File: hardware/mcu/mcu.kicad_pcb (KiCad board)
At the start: 2 copper layers, 24.5 x 68.8 mm, 61 parts, among them J1 TYPE-C-31-M-12, J2 Conn_01x11, J3 Conn_01x11, J4 JST-PH Battery, J5 n_log, Q1 MUN5214DW1T1G, Q2 SI2301CDS-T1-GE3, Q3 SI2301CDS-T1-GE3, Q4 SI2301CDS-T1-GE3, SW1 Reset, SW2 REG SELECT, SW3 Boot, U1 ESP32-PICO-D4, U2 CP210x, U3 USBLC6-2SC6, U4 TP4065, U5 ME6210A33P, U6 TPS630x1

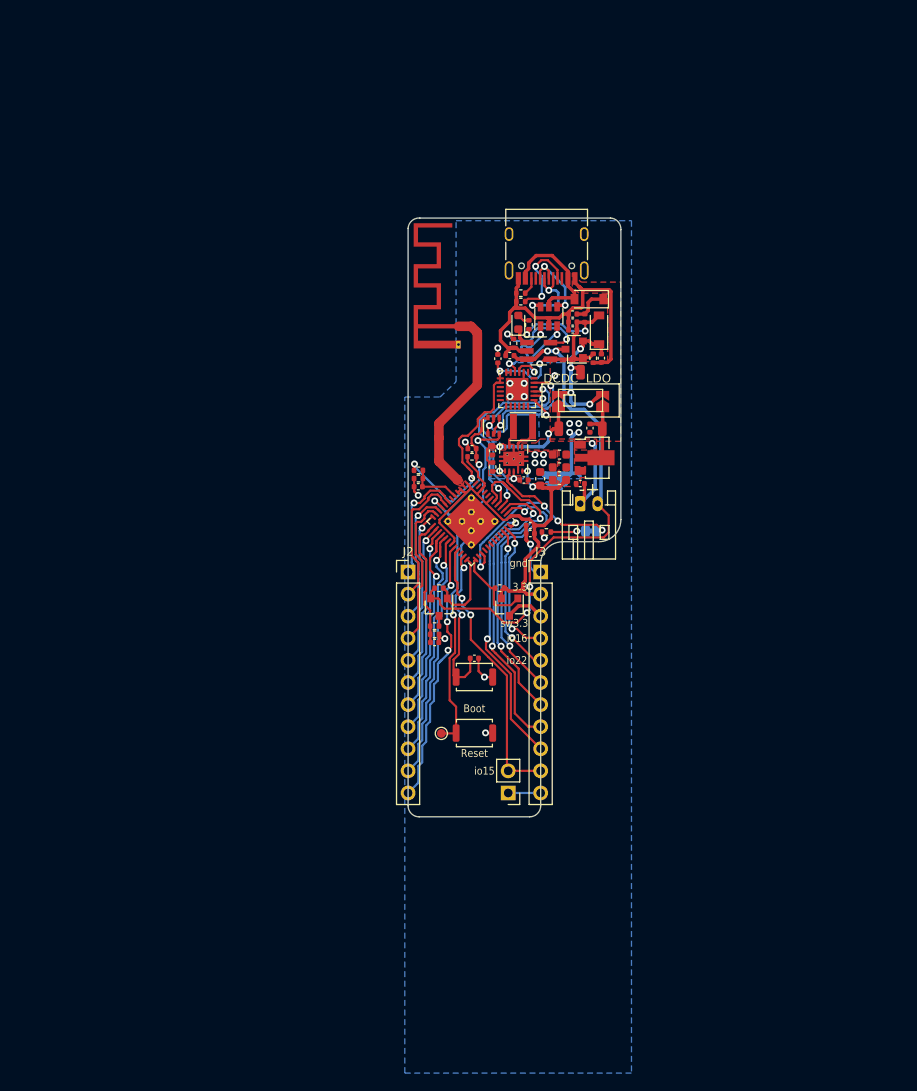
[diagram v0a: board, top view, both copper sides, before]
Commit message: Prototype scale v0.1
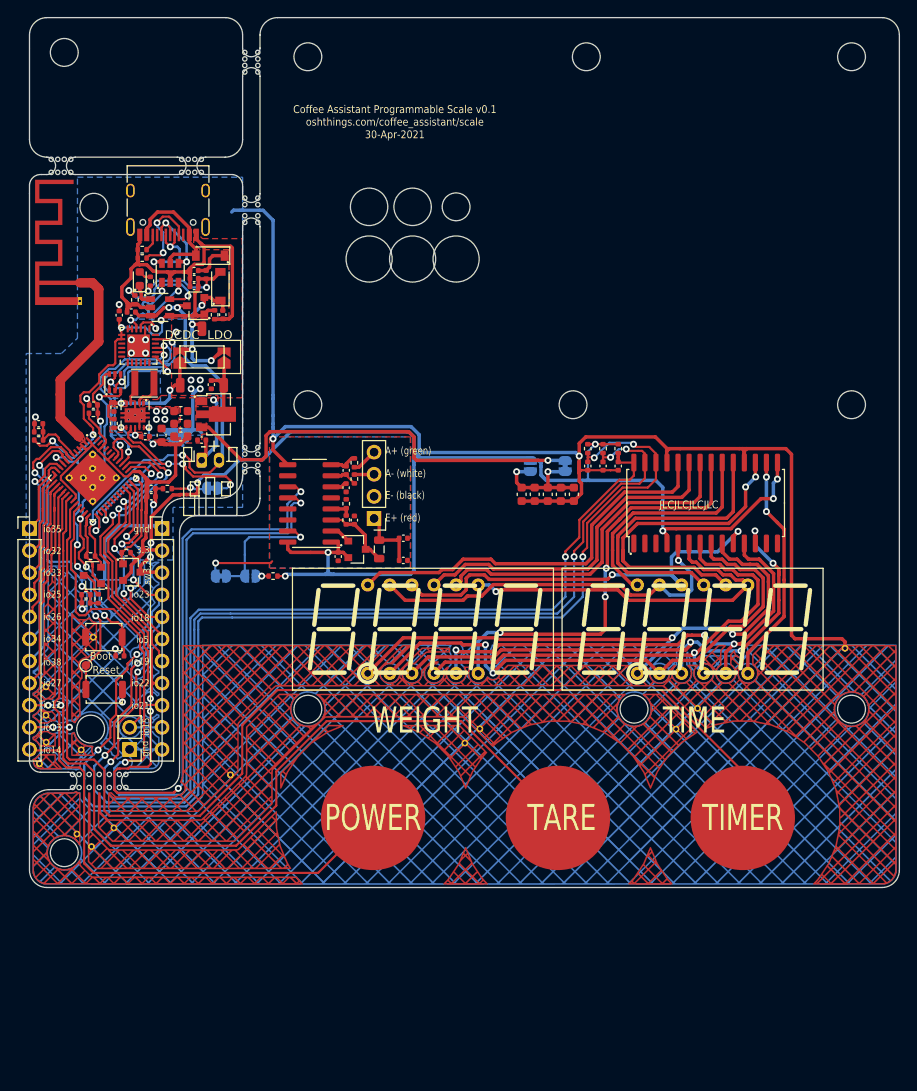
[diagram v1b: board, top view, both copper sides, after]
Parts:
- added C21: 10uF, Capacitor_SMD:C_0402_1005Metric, F.Cu at (93.5, 105.0)
- added C22: 10uF, Capacitor_SMD:C_0402_1005Metric, F.Cu at (95.3, 100.8)
- added C23: 100nF, Capacitor_SMD:C_0402_1005Metric, F.Cu at (94.4, 97.0)
- added C24: 100nF, Capacitor_SMD:C_0402_1005Metric, F.Cu at (94.4, 95.0)
- added C25: 100pF, Capacitor_SMD:C_0402_1005Metric, F.Cu at (122.2, 94.5)
- added C26: 100pF, Capacitor_SMD:C_0402_1005Metric, F.Cu at (123.9, 94.5)
- added C27: 100pF, Capacitor_SMD:C_0402_1005Metric, F.Cu at (125.7, 94.5)
- added C28: 22uF, Capacitor_SMD:C_0603_1608Metric, F.Cu at (119.1, 97.8)
- added C29: 22uF, Capacitor_SMD:C_0603_1608Metric, F.Cu at (114.6, 97.8)
- added C30: 22uF, Capacitor_SMD:C_0603_1608Metric, F.Cu at (117.6, 97.8)
- added C31: 22uF, Capacitor_SMD:C_0603_1608Metric, F.Cu at (120.6, 97.8)
- added C32: 22uF, Capacitor_SMD:C_0603_1608Metric, F.Cu at (116.1, 97.8)
- added C33: 100nF, Capacitor_SMD:C_0402_1005Metric, F.Cu at (101.0, 102.8)
- added C34: 10uF, Capacitor_SMD:C_0402_1005Metric, F.Cu at (101.0, 105.4)
- added CAP1: Power, custom:CapTouch_12mm, F.Cu at (97.5, 135.0)
- added CAP2: Tare, custom:CapTouch_12mm, F.Cu at (118.8, 135.0)
- added CAP3: Timer/Cal, custom:CapTouch_12mm, F.Cu at (140.0, 135.0)
- added CAP_GND_HATCHED_1: Cap sense grid ground, scale:cap_gnd_1_hatched, F.Cu at (65.7, 117.5)
- added CAP_GND_HATCHED_2: Cap sense grid ground, scale:cap_gnd_2_hatched, F.Cu at (108.0, 128.9)
- added CAP_GND_HATCHED_3: Cap sense grid ground, scale:cap_gnd_3_hatched, F.Cu at (62.0, 118.2)
- added CAP_GND_HATCHED_4: Cap sense grid ground, scale:cap_gnd_4_hatched, F.Cu at (108.0, 128.9)
- added J6: Conn_01x04, Connector_PinHeader_2.54mm:PinHeader_1x04_P2.54mm_Vertical, F.Cu at (97.6, 100.6)
- added JP2: extra_caps_nSwitched, Jumper:SolderJumper-2_P1.3mm_Bridged_RoundedPad1.0x1.5mm, B.Cu at (119.6, 94.5)
- added JP3: extra_caps_switched, Jumper:SolderJumper-2_P1.3mm_Open_RoundedPad1.0x1.5mm, B.Cu at (115.6, 94.5)
- added JP4: 80SPS, Jumper:SolderJumper-2_P1.3mm_Open_RoundedPad1.0x1.5mm, B.Cu at (83.4, 107.2)
- added JP5: 10SPS, Jumper:SolderJumper-2_P1.3mm_Bridged_RoundedPad1.0x1.5mm, B.Cu at (80.0, 107.2)
- added L2: 3.3uH, Inductor_SMD:L_0805_2012Metric, F.Cu at (98.2, 104.1)
- added Q5: SS8550, Package_TO_SOT_SMD:SOT-23, F.Cu at (95.7, 104.1)
- added R15: 100, Resistor_SMD:R_0402_1005Metric, F.Cu at (95.3, 96.0)
- added R16: 100, Resistor_SMD:R_0402_1005Metric, F.Cu at (95.3, 94.2)
- added R17: 20k, Resistor_SMD:R_0402_1005Metric, F.Cu at (94.4, 100.7)
- added R18: 8.2k, Resistor_SMD:R_0402_1005Metric, F.Cu at (94.4, 98.9)
- added R19: 10k, Resistor_SMD:R_0402_1005Metric, F.Cu at (122.2, 92.5)
- added R20: 10k, Resistor_SMD:R_0402_1005Metric, F.Cu at (123.9, 92.5)
- added R21: 10k, Resistor_SMD:R_0402_1005Metric, F.Cu at (125.7, 92.5)
- added R22: 10k, Resistor_SMD:R_0402_1005Metric, F.Cu at (86.0, 107.2)
- added REF**: MountingHole_3.2mm_M3_ISO7380_Pad, MountingHole:MountingHole_3.2mm_M3_ISO7380_Pad, F.Cu at (90.0, 122.5)
- added REF**: MountingHole_3.2mm_M3_ISO7380_Pad, MountingHole:MountingHole_3.2mm_M3_ISO7380_Pad, F.Cu at (65.0, 124.8)
- added REF**: MountingHole_3.2mm_M3_ISO7380_Pad, MountingHole:MountingHole_3.2mm_M3_ISO7380_Pad, F.Cu at (62.0, 139.0)
- added REF**: MountingHole_3.2mm_M3_ISO7380_Pad, MountingHole:MountingHole_3.2mm_M3_ISO7380_Pad, F.Cu at (152.5, 47.5)
- added REF**: MountingHole_3.2mm_M3_ISO7380_Pad, MountingHole:MountingHole_3.2mm_M3_ISO7380_Pad, F.Cu at (90.0, 47.5)
- added REF**: MountingHole_3.2mm_M3_ISO7380_Pad, MountingHole:MountingHole_3.2mm_M3_ISO7380_Pad, F.Cu at (65.4, 64.8)
- added REF**: MountingHole_3.2mm_M3_ISO7380_Pad, MountingHole:MountingHole_3.2mm_M3_ISO7380_Pad, F.Cu at (152.5, 122.5)
- added REF**: MountingHole_3.2mm_M3_ISO7380_Pad, MountingHole:MountingHole_3.2mm_M3_ISO7380_Pad, F.Cu at (127.5, 122.5)
- added REF**: MountingHole_3.2mm_M3_ISO7380_Pad, MountingHole:MountingHole_3.2mm_M3_ISO7380_Pad, F.Cu at (152.5, 87.5)
- added REF**: MountingHole_3.2mm_M3_ISO7380_Pad, MountingHole:MountingHole_3.2mm_M3_ISO7380_Pad, F.Cu at (122.0, 47.5)
- added REF**: MountingHole_3.2mm_M3_ISO7380_Pad, MountingHole:MountingHole_3.2mm_M3_ISO7380_Pad, F.Cu at (120.5, 87.5)
- added REF**: load_cell, custom:load_cell, F.Cu at (126.0, 67.5)
- added REF**: MountingHole_3.2mm_M3_ISO7380_Pad, MountingHole:MountingHole_3.2mm_M3_ISO7380_Pad, F.Cu at (62.0, 47.0)
- added REF**: MountingHole_3.2mm_M3_ISO7380_Pad, MountingHole:MountingHole_3.2mm_M3_ISO7380_Pad, F.Cu at (90.0, 87.5)
- added U10: FJ3461AH, custom:FJ3461AH, F.Cu at (134.2, 113.3)
- added U7: HX711, custom:SOP-16_3.9x9.9mm_P1.27mm, F.Cu at (90.2, 98.8)
- added U8: TM1638, Package_SO:SOIC-28W_7.5x17.9mm_P1.27mm, F.Cu at (135.7, 98.8)
- added U9: FJ3461AH, custom:FJ3461AH, F.Cu at (103.2, 113.3)
- added mouse-bite-single: VAL**, custom:mouse-bite-single, F.Cu at (84.2, 66.5)
- added mouse-bite-single: VAL**, custom:mouse-bite-single, F.Cu at (76.2, 60.8)
- added mouse-bite-single: VAL**, custom:mouse-bite-single, F.Cu at (75.5, 60.8)
- added mouse-bite-single: VAL**, custom:mouse-bite-single, F.Cu at (77.0, 59.3)
- added mouse-bite-single: VAL**, custom:mouse-bite-single, F.Cu at (76.2, 59.3)
- added mouse-bite-single: VAL**, custom:mouse-bite-single, F.Cu at (68.3, 130.0)
- added mouse-bite-single: VAL**, custom:mouse-bite-single, F.Cu at (68.3, 131.5)
- added mouse-bite-single: VAL**, custom:mouse-bite-single, F.Cu at (62.8, 59.3)
- added mouse-bite-single: VAL**, custom:mouse-bite-single, F.Cu at (62.8, 60.8)
- added mouse-bite-single: VAL**, custom:mouse-bite-single, F.Cu at (61.2, 59.3)
- added mouse-bite-single: VAL**, custom:mouse-bite-single, F.Cu at (60.5, 59.3)
- added mouse-bite-single: VAL**, custom:mouse-bite-single, F.Cu at (84.2, 65.8)
- added mouse-bite-single: VAL**, custom:mouse-bite-single, F.Cu at (62.0, 60.8)
- added mouse-bite-single: VAL**, custom:mouse-bite-single, F.Cu at (61.2, 60.8)
- added mouse-bite-single: VAL**, custom:mouse-bite-single, F.Cu at (60.5, 60.8)
- added mouse-bite-single: VAL**, custom:mouse-bite-single, F.Cu at (62.0, 59.3)
- added mouse-bite-single: VAL**, custom:mouse-bite-single, F.Cu at (84.2, 48.5)
- added mouse-bite-single: VAL**, custom:mouse-bite-single, F.Cu at (84.2, 49.2)
- added mouse-bite-single: VAL**, custom:mouse-bite-single, F.Cu at (82.8, 47.8)
- added mouse-bite-single: VAL**, custom:mouse-bite-single, F.Cu at (82.8, 48.5)
- added mouse-bite-single: VAL**, custom:mouse-bite-single, F.Cu at (82.8, 49.2)
- added mouse-bite-single: VAL**, custom:mouse-bite-single, F.Cu at (84.2, 47.8)
- added mouse-bite-single: VAL**, custom:mouse-bite-single, F.Cu at (82.8, 64.5)
- added mouse-bite-single: VAL**, custom:mouse-bite-single, F.Cu at (82.8, 47.0)
- added mouse-bite-single: VAL**, custom:mouse-bite-single, F.Cu at (84.2, 47.0)
- added mouse-bite-single: VAL**, custom:mouse-bite-single, F.Cu at (66.0, 131.5)
- added mouse-bite-single: VAL**, custom:mouse-bite-single, F.Cu at (66.0, 130.0)
- added mouse-bite-single: VAL**, custom:mouse-bite-single, F.Cu at (64.9, 130.0)
- added mouse-bite-single: VAL**, custom:mouse-bite-single, F.Cu at (64.9, 131.5)
- added mouse-bite-single: VAL**, custom:mouse-bite-single, F.Cu at (84.2, 64.5)
- added mouse-bite-single: VAL**, custom:mouse-bite-single, F.Cu at (82.8, 63.8)
- added mouse-bite-single: VAL**, custom:mouse-bite-single, F.Cu at (84.2, 63.8)
- added mouse-bite-single: VAL**, custom:mouse-bite-single, F.Cu at (82.8, 95.2)
- added mouse-bite-single: VAL**, custom:mouse-bite-single, F.Cu at (82.8, 65.8)
- added mouse-bite-single: VAL**, custom:mouse-bite-single, F.Cu at (84.2, 93.2)
- added mouse-bite-single: VAL**, custom:mouse-bite-single, F.Cu at (82.8, 93.2)
- added mouse-bite-single: VAL**, custom:mouse-bite-single, F.Cu at (84.2, 94.5)
- added mouse-bite-single: VAL**, custom:mouse-bite-single, F.Cu at (82.8, 94.5)
- added mouse-bite-single: VAL**, custom:mouse-bite-single, F.Cu at (84.2, 95.2)
- added mouse-bite-single: VAL**, custom:mouse-bite-single, F.Cu at (82.8, 92.4)
- added mouse-bite-single: VAL**, custom:mouse-bite-single, F.Cu at (84.2, 92.4)
- added mouse-bite-single: VAL**, custom:mouse-bite-single, F.Cu at (63.7, 131.5)
- added mouse-bite-single: VAL**, custom:mouse-bite-single, F.Cu at (63.0, 131.5)
- added mouse-bite-single: VAL**, custom:mouse-bite-single, F.Cu at (67.2, 130.0)
- added mouse-bite-single: VAL**, custom:mouse-bite-single, F.Cu at (82.8, 66.5)
- added mouse-bite-single: VAL**, custom:mouse-bite-single, F.Cu at (63.7, 130.0)
- added mouse-bite-single: VAL**, custom:mouse-bite-single, F.Cu at (63.0, 130.0)
- added mouse-bite-single: VAL**, custom:mouse-bite-single, F.Cu at (67.2, 131.5)
- added mouse-bite-single: VAL**, custom:mouse-bite-single, F.Cu at (69.1, 130.0)
- added mouse-bite-single: VAL**, custom:mouse-bite-single, F.Cu at (69.1, 131.5)
- added mouse-bite-single: VAL**, custom:mouse-bite-single, F.Cu at (77.0, 60.8)
- added mouse-bite-single: VAL**, custom:mouse-bite-single, F.Cu at (75.5, 59.3)
- added mouse-bite-single: VAL**, custom:mouse-bite-single, F.Cu at (77.8, 60.8)
- added mouse-bite-single: VAL**, custom:mouse-bite-single, F.Cu at (77.8, 59.3)
- R5: value 3k -> 3.3k
- SW1: value Reset -> SKRKAEE020
- SW3: value Boot -> SKRKAEE020
- U4: footprint Package_TO_SOT_SMD:SOT-23-5_HandSoldering -> Package_TO_SOT_SMD:SOT-23-5
- moved C20 44.2 mm to (59.1, 89.7)
- moved R13 44.0 mm to (59.1, 90.6)
- moved C18 43.9 mm to (72.0, 97.1), turned to 180 degrees
- moved R14 43.9 mm to (73.8, 97.2)
- moved C15 43.8 mm to (73.2, 91.0)
- moved C6 43.8 mm to (65.3, 87.5)
- moved D1 43.8 mm to (78.8, 70.4)
- moved D3 43.8 mm to (70.7, 73.0)
- moved FB1 43.8 mm to (78.3, 72.5)
- moved J3 43.8 mm to (73.2, 101.7)
- moved L1 43.8 mm to (71.2, 85.0)
- moved R1 43.8 mm to (71.0, 70.6)
- moved R2 43.8 mm to (71.0, 69.7)
- moved R3 43.8 mm to (79.3, 77.2)
- moved R6 43.8 mm to (65.3, 88.5)
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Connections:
- net /SWITCHED_3v3 renamed SWITCHED_3v3
- C20 pad 2: /sensor_vp -> /sensor_capp
- J2 pad 1: /sensor_capn -> /io35
- J2 pad 10: /io12 -> /io13
- J2 pad 11: /io13 -> /io14
- J2 pad 2: /sensor_vn -> /io32
- J2 pad 3: /io34 -> /io33
- J2 pad 4: /io35 -> /io25
- J2 pad 5: /io32 -> /io26
- J2 pad 6: /io25 -> /io34
- J2 pad 7: /io26 -> /sensor_capn
- J2 pad 9: /io14 -> /io12
- J3 pad 4: /io18 -> /io23
- J3 pad 5: /io5 -> /io18
- J3 pad 6: /io19 -> /io5
- J3 pad 7: /io21 -> /io19
- J3 pad 9: /io23 -> /io21
- R12 pad 1: /sensor_vp -> /sensor_capp
- R13 pad 2: /sensor_vp -> /sensor_capp
- U1 pad 13: /batt_adc -> /io33
- U1 pad 8: /sensor_vn -> /batt_adc
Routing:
- net GND: track 26.5 -> 432.4 mm, vias 8 -> 10
- net SWITCHED_3v3: track 4.52 -> 157.3 mm, vias 0 -> 9
- net /io18: track 15.8 -> 147.7 mm, vias 2 -> 7
- net /io23: track 31.2 -> 157.7 mm, vias 2 -> 7
- net /io5: track 16.9 -> 137.8 mm, vias 2 -> 5
- net /io13: track 30.8 -> 139.3 mm, vias 3 -> 2
- net /io12: track 28.0 -> 113.7 mm, vias 1 -> 2
- net /io21: track 38.0 -> 115.1 mm, vias 2 -> 4
- net /io22: track 34.5 -> 109.3 mm, vias 2 -> 6
- net /scale/e: track 0.00 -> 66.9 mm, vias 0 -> 2
- net /scale/d: track 0.00 -> 63.4 mm, vias 0 -> 2
- net /scale/dp: track 0.00 -> 63.4 mm, vias 0 -> 4
- net /io14: track 27.2 -> 86.5 mm, vias 1 -> 0
- net /scale/g: track 0.00 -> 56.0 mm, vias 0 -> 3
- net /scale/c: track 0.00 -> 55.6 mm, vias 0 -> 1
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- added copper zone on F.Cu, net GND
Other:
- board size 24.5 x 68.8 mm -> 100 x 100 mm
- rule pad_to_mask_clearance: 0.05 -> 0
- board text added: "10"
- board text added: "80"
- board text added: "80 is noisier don't bridge both..."
- board text added: "A+ (green)"
- board text added: "A- (white)"
- board text added: "Coffee Assistant Programmable Scale v0.1 oshthings.com/coffee_assistant/scale 30-Apr-2021"
- board text added: "E+ (red)"
- board text added: "E- (black)"
- board text added: "JLCJLCJLCJLC"
- board text added: "POWER"
- board text added: "TARE"
- board text added: "TIME"
- board text added: "TIMER"
- board text added: "WEIGHT"
- board text added: "cut to float dcdc powersave pin"
- board text added: "extra capacitance"
- board text added: "extra capacitance on sw may cause brown out"
- board text added: "io12"
- board text added: "io13"
- board text added: "io14"
- board text added: "io18"
- board text added: "io19"
- board text added: "io21"
- board text added: "io23"
- board text added: "io25"
- board text added: "io26"
- board text added: "io27"
- board text added: "io32"
- board text added: "io33"
- board text added: "io34"
- board text added: "io35"
- board text added: "io38"
- board text added: "io5"
- board text added: "jumper to silence boot log"
- board text added: "rate (samp/s)"
- board text added: "sw3.3 is switched 3.3 attached to io16 defaults to disabled"
- board text removed: "io16"
